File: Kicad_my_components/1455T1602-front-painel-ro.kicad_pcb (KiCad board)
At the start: 2 copper layers, 165 x 51.5 mm, 0 parts

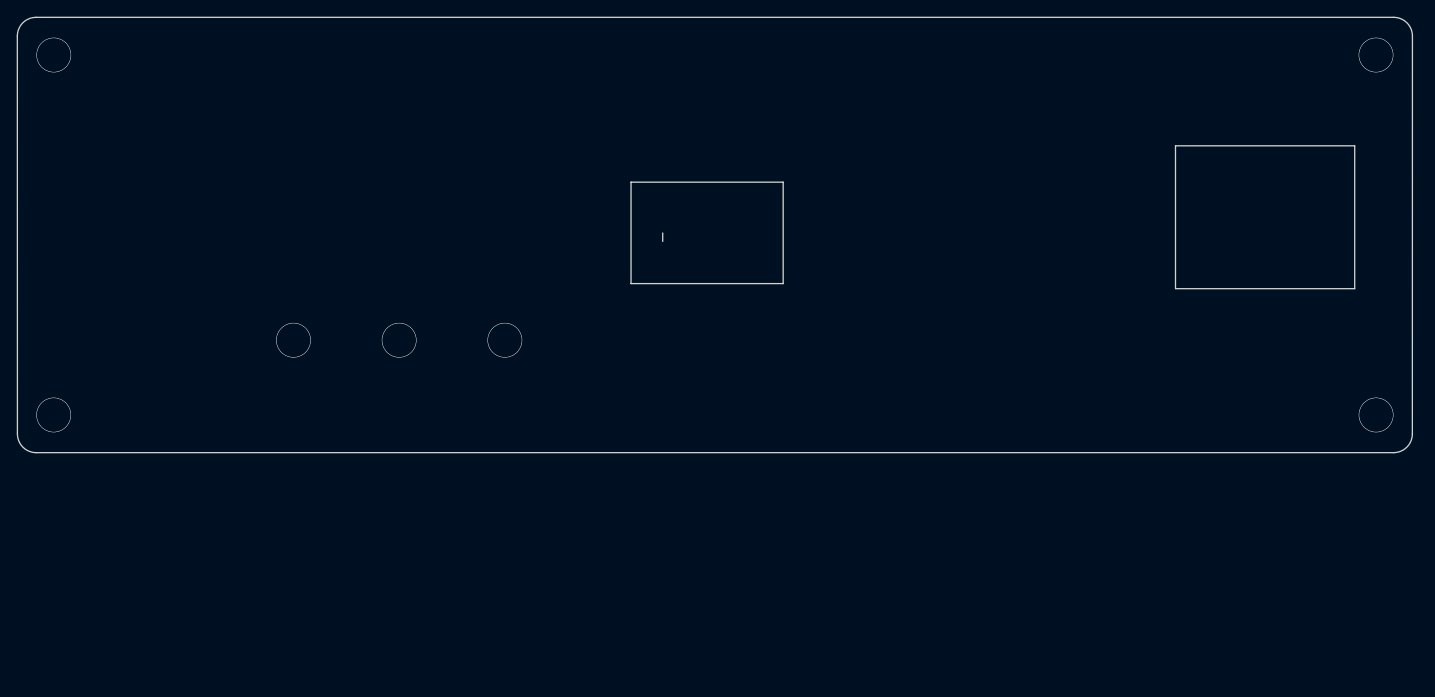
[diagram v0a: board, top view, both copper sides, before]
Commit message: Fixed all
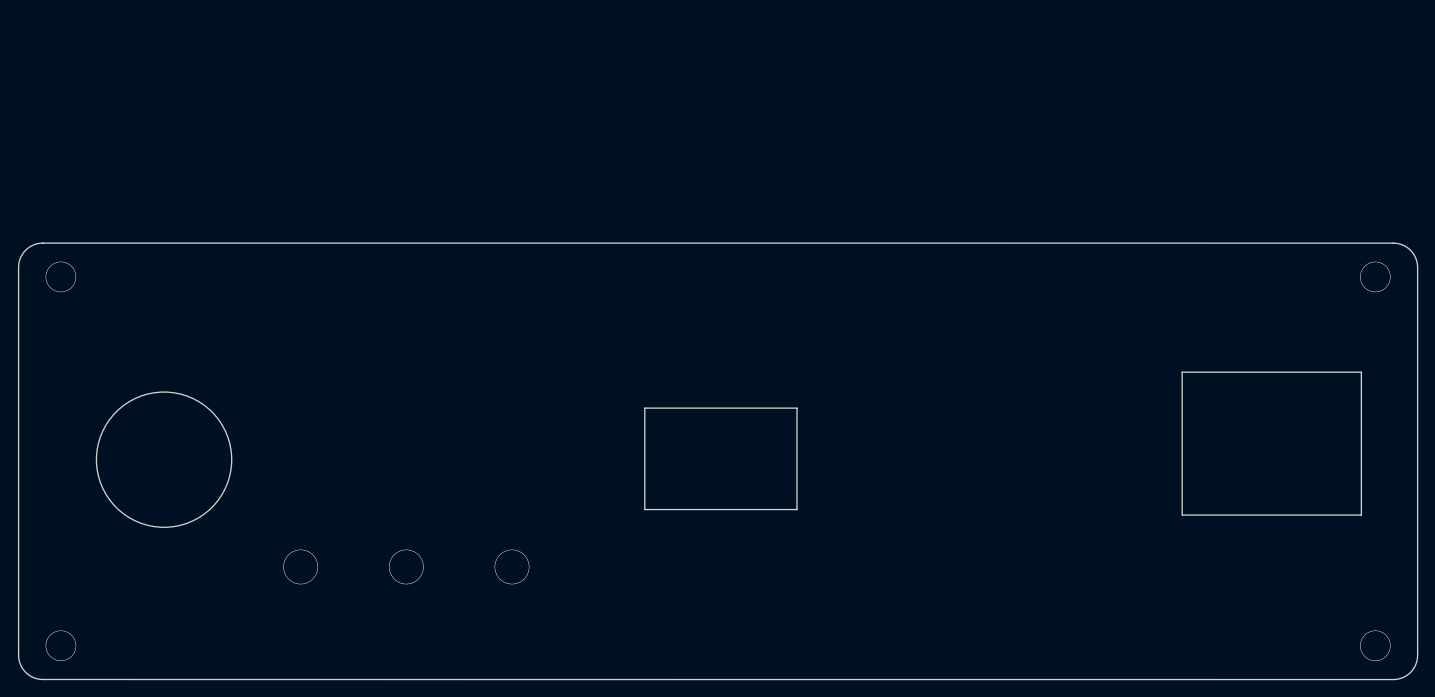
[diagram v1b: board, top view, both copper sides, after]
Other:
- board size 165 x 51.5 mm -> 165.5 x 51.6 mm
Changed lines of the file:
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@@
       (drillshape 0)
       (scaleselection 1)
-      (outputdirectory "gbr2/")
+      (outputdirectory "E:/painel 1/")
     )
   )
   (net 0 "")
-  (gr_circle (center 85.02 74.03) (end 93.02 74.03) (layer "Dwgs.User") (width 0.15) (fill none))
-  (gr_line (start 68.97009 100.02) (end 229.54991 100.02) (layer "Edge.Cuts") (width 0.1))
-  (gr_arc (start 231.76991 97.8) (mid 231.119687 99.369777) (end 229.54991 100.02) (layer "Edge.Cuts") (width 0.1))
-  (gr_line (start 224.95 80.62) (end 224.95 63.72) (layer "Edge.Cuts") (width 0.1))
-  (gr_arc (start 229.55991 48.52) (mid 231.129751 49.170249) (end 231.78 50.74009) (layer "Edge.Cuts") (width 0.1))
-  (gr_arc (start 68.97009 100.02) (mid 67.400313 99.369777) (end 66.75009 97.8) (layer "Edge.Cuts") (width 0.1))
-  (gr_line (start 68.96009 48.52) (end 229.55991 48.52) (layer "Edge.Cuts") (width 0.1))
-  (gr_line (start 231.77991 50.74) (end 231.76991 97.8) (layer "Edge.Cuts") (width 0.1))
-  (gr_line (start 139.34 68.02) (end 157.34 68.02) (layer "Edge.Cuts") (width 0.1))
-  (gr_line (start 203.77 80.62) (end 224.95 80.62) (layer "Edge.Cuts") (width 0.1))
-  (gr_arc (start 66.74 50.74009) (mid 67.390249 49.170249) (end 68.96009 48.52) (layer "Edge.Cuts") (width 0.1))
-  (gr_line (start 66.75009 97.8) (end 66.74009 50.74) (layer "Edge.Cuts") (width 0.1))
-  (gr_line (start 157.34 68.02) (end 157.34 80.02) (layer "Edge.Cuts") (width 0.1))
-  (gr_line (start 143.09 75.03) (end 143.09 74.03) (layer "Edge.Cuts") (width 0.1))
-  (gr_line (start 203.75 63.72) (end 203.75 80.62) (layer "Edge.Cuts") (width 0.1))
-  (gr_line (start 157.34 80.02) (end 139.34 80.02) (layer "Edge.Cuts") (width 0.1))
-  (gr_line (start 139.34 80.02) (end 139.34 68.02) (layer "Edge.Cuts") (width 0.1))
-  (gr_line (start 224.95 63.72) (end 203.75 63.72) (layer "Edge.Cuts") (width 0.1))
-  (gr_text "R8" (at 187.51 49.39 180) (layer "F.Fab")
+  (gr_arc (start 229.518529 75.231471) (mid 231.550006 76.072936) (end 232.391471 78.104413) (layer "Edge.Cuts") (width 0.1))
+  (gr_line (start 232.391471 78.104413) (end 232.391471 123.988529) (layer "Edge.Cuts") (width 0.1))
+  (gr_line (start 225.74 107.4) (end 225.74 90.5) (layer "Edge.Cuts") (width 0.1))
+  (gr_arc (start 69.764413 126.854413) (mid 67.732936 126.012948) (end 66.891471 123.981471) (layer "Edge.Cuts") (width 0.1))
+  (gr_line (start 69.761471 75.228529) (end 229.518529 75.231471) (layer "Edge.Cuts") (width 0.1))
+  (gr_line (start 140.97 94.75) (end 158.97 94.75) (layer "Edge.Cuts") (width 0.1))
+  (gr_line (start 229.518529 126.861471) (end 69.764413 126.854413) (layer "Edge.Cuts") (width 0.1))
+  (gr_line (start 204.56 107.4) (end 225.74 107.4) (layer "Edge.Cuts") (width 0.1))
+  (gr_line (start 66.891471 123.981471) (end 66.888529 78.101471) (layer "Edge.Cuts") (width 0.1))
+  (gr_line (start 158.97 94.75) (end 158.97 106.75) (layer "Edge.Cuts") (width 0.1))
+  (gr_line (start 204.54 90.5) (end 204.54 107.4) (layer "Edge.Cuts") (width 0.1))
+  (gr_line (start 158.97 106.75) (end 140.97 106.75) (layer "Edge.Cuts") (width 0.1))
+  (gr_circle (center 84.1 100.85) (end 92.1 100.85) (layer "Edge.Cuts") (width 0.15) (fill none))
+  (gr_arc (start 232.391471 123.988529) (mid 231.550006 126.020006) (end 229.518529 126.861471) (layer "Edge.Cuts") (width 0.1))
+  (gr_line (start 140.97 106.75) (end 140.97 94.75) (layer "Edge.Cuts") (width 0.1))
+  (gr_line (start 225.74 90.5) (end 204.54 90.5) (layer "Edge.Cuts") (width 0.1))
+  (gr_arc (start 66.888529 78.101471) (mid 67.729994 76.069994) (end 69.761471 75.228529) (layer "Edge.Cuts") (width 0.1))
+  (gr_text "R8" (at 187.891471 76.227942 180) (layer "F.Fab")
     (effects (font (size 0.5 0.5) (thickness 0.08)))
   )
-  (segment (start 227.47 95.55009) (end 227.48 95.56009) (width 0.25) (layer "F.Cu") (net 0))
-  (via (at 71.04 95.56009) (size 4.1) (drill 4) (layers "F.Cu" "B.Cu") (free) (net 0))
-  (via (at 227.48 95.56009) (size 4.1) (drill 4) (layers "F.Cu" "B.Cu") (free) (net 0))
-  (via (at 124.41 86.72) (size 4.1) (drill 4) (layers "F.Cu" "B.Cu") (free) (net 0))
-  (via (at 99.41 86.72) (size 4.1) (drill 4) (layers "F.Cu" "B.Cu") (free) (net 0))
-  (via (at 227.47 52.98) (size 4.1) (drill 4) (layers "F.Cu" "B.Cu") (free) (net 0))
-  (via (at 111.91 86.72) (size 4.1) (drill 4) (layers "F.Cu" "B.Cu") (free) (net 0))
-  (via (at 71.05 52.98) (size 4.1) (drill 4) (layers "F.Cu" "B.Cu") (free) (net 0))
-  (segment (start 71.05 95.55009) (end 71.04 95.56009) (width 0.25) (layer "B.Cu") (net 0))
+  (via (at 125.26 113.54) (size 4.1) (drill 4) (layers "F.Cu" "B.Cu") (free) (net 0))
+  (via (at 100.26 113.54) (size 4.1) (drill 4) (layers "F.Cu" "B.Cu") (free) (net 0))
+  (via (at 227.391471 122.861471) (size 3.6) (drill 3.5) (layers "F.Cu" "B.Cu") (free) (net 0))
+  (via (at 112.76 113.54) (size 4.1) (drill 4) (layers "F.Cu" "B.Cu") (free) (net 0))
+  (via (at 71.891471 79.231471) (size 3.6) (drill 3.5) (layers "F.Cu" "B.Cu") (free) (net 0))
+  (via (at 227.391471 79.231471) (size 3.6) (drill 3.5) (layers "F.Cu" "B.Cu") (free) (net 0))
+  (via (at 71.891471 122.861471) (size 3.6) (drill 3.5) (layers "F.Cu" "B.Cu") (free) (net 0))
 )
